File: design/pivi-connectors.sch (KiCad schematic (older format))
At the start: 15 parts, among them P2 External 5v, P3 Recom_Power_RAC10-05SC/277, P4 CONN_01X04, P5 CONN_02X20, P6 Debug uart

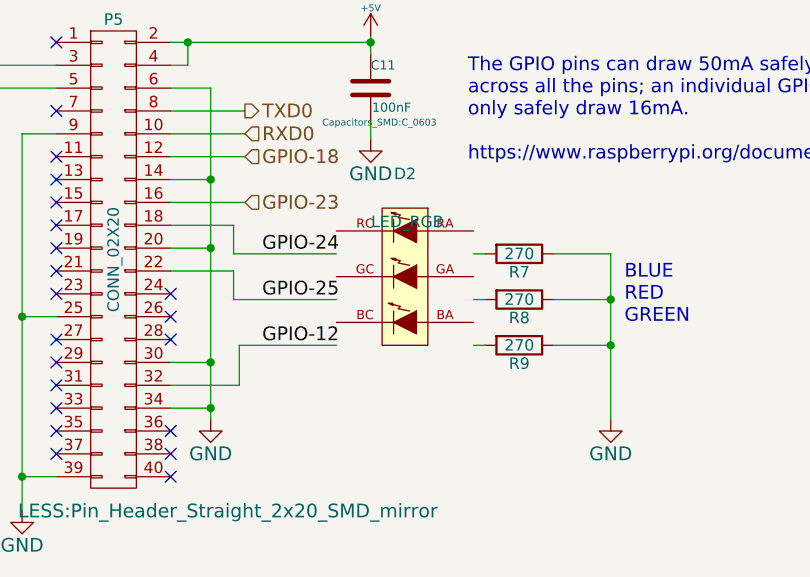
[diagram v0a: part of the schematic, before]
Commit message: PIVI version 2.1 routed.
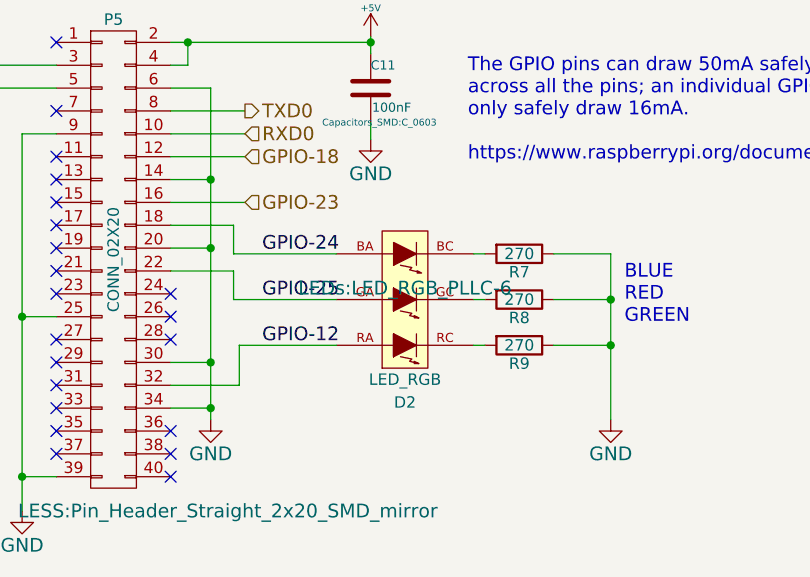
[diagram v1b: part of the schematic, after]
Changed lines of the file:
@@
 LIBS:txs0104e
 LIBS:less
+LIBS:RGB-LED-PLL6
 EELAYER 25 0
 EELAYER END
@@
 GPIO-23
 $Comp
-L LED_RGB D2
-U 1 1 55BA51D0
-P 8540 2290
-F 0 "D2" H 8540 2740 50  0000 C CNN
-F 1 "LED_RGB" H 8550 2530 50  0000 C CNN
-F 2 "LEDs:LED_RGB_PLLC-6" H 8540 2240 60  0001 C CNN
-F 3 "" H 8540 2240 60  0000 C CNN
-	1    8540 2290
-	1    0    0    -1
-$EndComp
-$Comp
 L R R7
 U 1 1 55BA6452
@@
 Text Notes 9500 2500 0    60   ~ 0
 BLUE\nRED\nGREEN
+$Comp
+L LED_RGB D2
+U 1 1 55F5FF1D
+P 8540 2390
+F 0 "D2" H 8540 2840 50  0000 C CNN
+F 1 "LED_RGB" H 8540 2740 50  0000 C CNN
+F 2 "LEDs:LED_RGB_PLLC-6" H 8540 2340 60  0000 C CNN
+F 3 "" H 8540 2340 60  0000 C CNN
+	1    8540 2390
+	-1   0    0    1
+$EndComp
 $EndSCHEMATC
